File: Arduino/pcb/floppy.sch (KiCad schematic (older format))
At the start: 11 parts, among them J7 Floppy-Power, J8 IBM_PC_Floppy_IDC, SW1 Bus Address Select, U1 4021

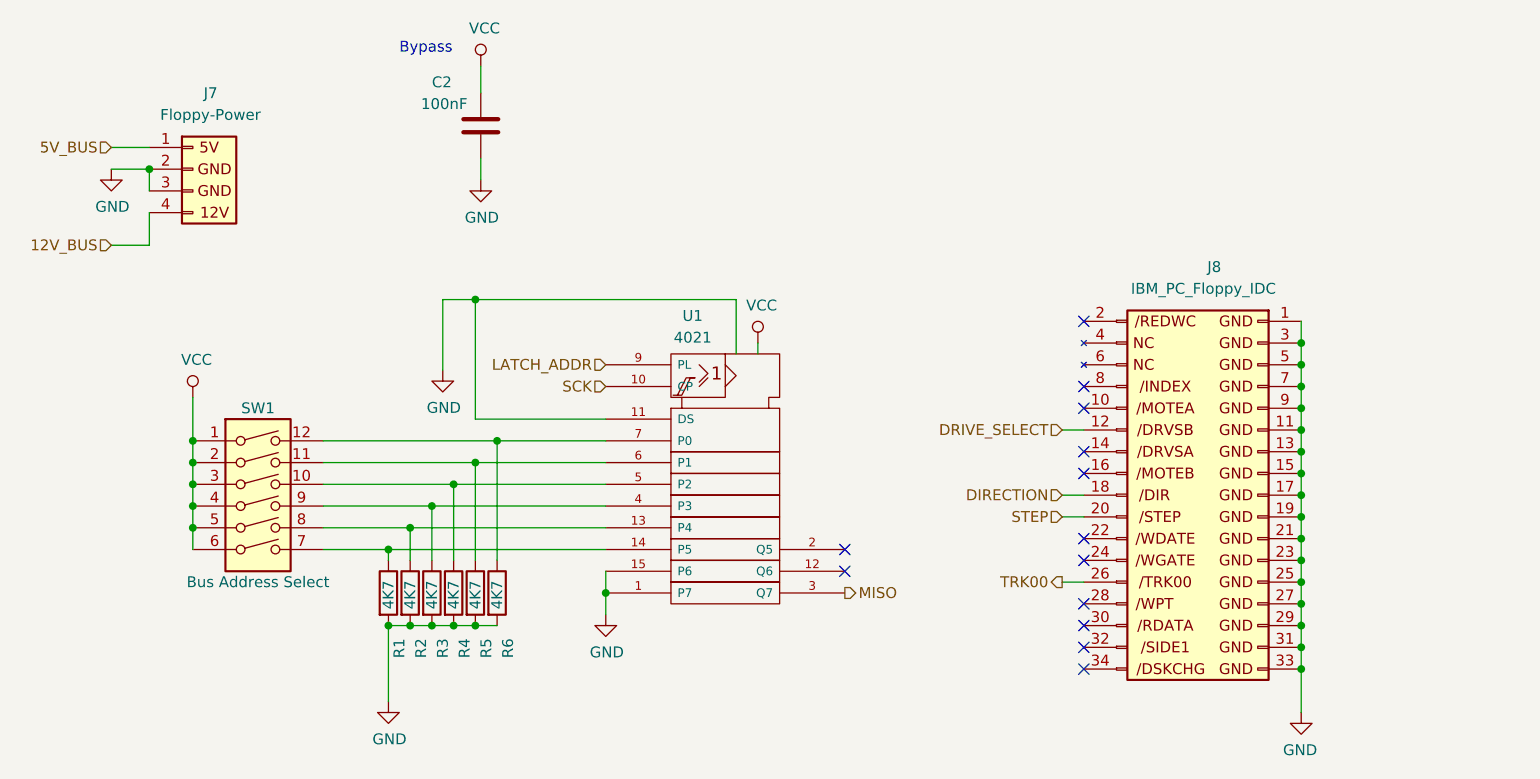
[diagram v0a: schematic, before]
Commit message: pcb: did... something
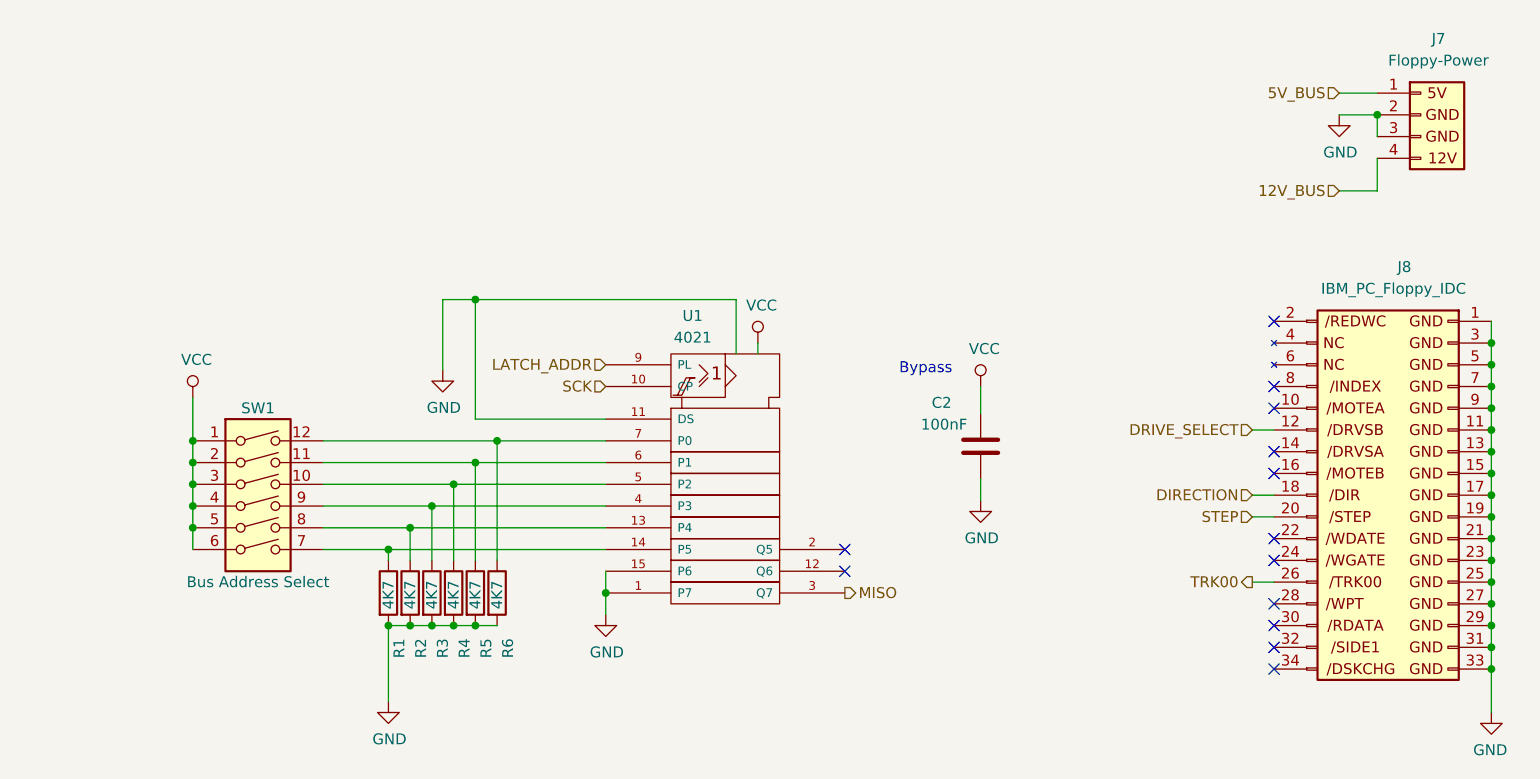
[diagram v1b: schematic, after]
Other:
- moved on the sheet: C2, J7, J8
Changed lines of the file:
@@
 Comment4 ""
 $EndDescr
-NoConn ~ 6075 2925
-NoConn ~ 6075 3025
-NoConn ~ 6075 3325
-NoConn ~ 6075 3625
-NoConn ~ 6075 3725
-NoConn ~ 6075 3925
-NoConn ~ 6075 4025
-NoConn ~ 6075 4125
-NoConn ~ 6075 4225
-NoConn ~ 6075 2625
-NoConn ~ 6075 3225
+NoConn ~ 6950 2925
+NoConn ~ 6950 3025
+NoConn ~ 6950 3325
+NoConn ~ 6950 3625
+NoConn ~ 6950 3725
+NoConn ~ 6950 3925
+NoConn ~ 6950 4025
+NoConn ~ 6950 4125
+NoConn ~ 6950 4225
+NoConn ~ 6950 2625
+NoConn ~ 6950 3225
 $Comp
 L ibm_pc_floppy_idc:IBM_PC_Floppy_IDC J?
 U 1 1 5CE26438
-P 6875 3425
+P 7750 3425
 AR Path="/5CE26438" Ref="J?"  Part="1"
 AR Path="/5CD0EE48/5CE26438" Ref="J8"  Part="1"
-F 0 "J8" H 7075 4475 50  0000 C CNN
-F 1 "IBM_PC_Floppy_IDC" H 7125 4375 50  0000 C CNN
-F 2 "ibm_idc_floppy_connector:ibm_pc_floppy_idc" H 6875 3425 50  0001 C CNN
-F 3 "" H 6875 3425 50  0001 C CNN
-	1    6875 3425
+F 0 "J8" H 7950 4475 50  0000 C CNN
+F 1 "IBM_PC_Floppy_IDC" H 8000 4375 50  0000 C CNN
+F 2 "ibm_idc_floppy_connector:ibm_pc_floppy_idc" H 7750 3425 50  0001 C CNN
+F 3 "" H 7750 3425 50  0001 C CNN
+	1    7750 3425
 	-1   0    0    -1
 $EndComp
 Wire Wire Line
-	7075 2625 7075 2725
-Connection ~ 7075 2725
-Wire Wire Line
-	7075 2725 7075 2825
-Connection ~ 7075 2825
-Wire Wire Line
-	7075 2825 7075 2925
-Connection ~ 7075 2925
-Wire Wire Line
-	7075 2925 7075 3025
-Connection ~ 7075 3025
-Wire Wire Line
-	7075 3025 7075 3125
-Connection ~ 7075 3125
-Wire Wire Line
-	7075 3125 7075 3225
-Connection ~ 7075 3225
-Wire Wire Line
-	7075 3225 7075 3325
-Connection ~ 7075 3325
-Wire Wire Line
-	7075 3325 7075 3425
-Connection ~ 7075 3425
-Wire Wire Line
-	7075 3425 7075 3525
-Connection ~ 7075 3525
-Wire Wire Line
-	7075 3525 7075 3625
-Connection ~ 7075 3625
-Wire Wire Line
-	7075 3625 7075 3725
-Connection ~ 7075 3725
-Wire Wire Line
-	7075 3725 7075 3825
-Connection ~ 7075 3825
-Wire Wire Line
-	7075 3825 7075 3925
-Connection ~ 7075 3925
-Wire Wire Line
-	7075 3925 7075 4025
-Connection ~ 7075 4025
-Wire Wire Line
-	7075 4025 7075 4125
-Wire Wire Line
-	7075 4125 7075 4225
-Connection ~ 7075 4125
-Connection ~ 7075 4225
-Wire Wire Line
-	7075 4225 7075 4425
+	7950 2625 7950 2725
+Connection ~ 7950 2725
+Wire Wire Line
+	7950 2725 7950 2825
+Connection ~ 7950 2825
+Wire Wire Line
+	7950 2825 7950 2925
+Connection ~ 7950 2925
+Wire Wire Line
+	7950 2925 7950 3025
+Connection ~ 7950 3025
+Wire Wire Line
+	7950 3025 7950 3125
+Connection ~ 7950 3125
+Wire Wire Line
+	7950 3125 7950 3225
+Connection ~ 7950 3225
+Wire Wire Line
+	7950 3225 7950 3325
+Connection ~ 7950 3325
+Wire Wire Line
+	7950 3325 7950 3425
+Connection ~ 7950 3425
+Wire Wire Line
+	7950 3425 7950 3525
+Connection ~ 7950 3525
+Wire Wire Line
+	7950 3525 7950 3625
+Connection ~ 7950 3625
+Wire Wire Line
+	7950 3625 7950 3725
+Connection ~ 7950 3725
+Wire Wire Line
+	7950 3725 7950 3825
+Connection ~ 7950 3825
+Wire Wire Line
+	7950 3825 7950 3925
+Connection ~ 7950 3925
+Wire Wire Line
+	7950 3925 7950 4025
+Connection ~ 7950 4025
+Wire Wire Line
+	7950 4025 7950 4125
+Wire Wire Line
+	7950 4125 7950 4225
+Connection ~ 7950 4125
+Connection ~ 7950 4225
+Wire Wire Line
+	7950 4225 7950 4425
 $Comp
 L power:GND #PWR?
 U 1 1 5CE2645F
-P 7075 4425
+P 7950 4425
 AR Path="/5CE2645F" Ref="#PWR?"  Part="1"
 AR Path="/5CD0EE48/5CE2645F" Ref="#PWR018"  Part="1"
-F 0 "#PWR018" H 7075 4175 50  0001 C CNN
-F 1 "GND" H 7080 4252 50  0000 C CNN
-F 2 "" H 7075 4425 50  0001 C CNN
-F 3 "" H 7075 4425 50  0001 C CNN
-	1    7075 4425
+F 0 "#PWR018" H 7950 4175 50  0001 C CNN
+F 1 "GND" H 7955 4252 50  0000 C CNN
+F 2 "" H 7950 4425 50  0001 C CNN
+F 3 "" H 7950 4425 50  0001 C CNN
+	1    7950 4425
 	-1   0    0    -1
 $EndComp
-Text HLabel 5975 3125 0    50   Input ~ 0
+Text HLabel 6850 3125 0    50   Input ~ 0
 DRIVE_SELECT
-Text HLabel 5975 3425 0    50   Input ~ 0
+Text HLabel 6850 3425 0    50   Input ~ 0
 DIRECTION
-Text HLabel 5975 3825 0    50   Output ~ 0
+Text HLabel 6850 3825 0    50   Output ~ 0
 TRK00
-Text HLabel 5975 3525 0    50   Input ~ 0
+Text HLabel 6850 3525 0    50   Input ~ 0
 STEP
 Wire Wire Line
-	5975 3125 6075 3125
-Wire Wire Line
-	5975 3425 6075 3425
-Wire Wire Line
-	5975 3525 6075 3525
-Wire Wire Line
-	5975 3825 6075 3825
+	6850 3125 6950 3125
+Wire Wire Line
+	6850 3425 6950 3425
+Wire Wire Line
+	6850 3525 6950 3525
+Wire Wire Line
+	6850 3825 6950 3825
 $Comp
 L floppy-power:Floppy-Power J?
 U 1 1 5CEBDDC6
-P 1975 1925
+P 7625 1675
 AR Path="/5CEBDDC6" Ref="J?"  Part="1"
 AR Path="/5CD0EE48/5CEBDDC6" Ref="J7"  Part="1"
-F 0 "J7" H 2025 2275 50  0000 L CNN
-F 1 "Floppy-Power" H 1825 2175 50  0000 L CNN
-F 2 "floppy_power:Floppy_Power_1x04_Pitch2.54mm" H 1975 1925 50  0001 C CNN
-F 3 "" H 1975 1925 50  0001 C CNN
-	1    1975 1925
+F 0 "J7" H 7675 2025 50  0000 L CNN
+F 1 "Floppy-Power" H 7475 1925 50  0000 L CNN
+F 2 "floppy_power:Floppy_Power_1x04_Pitch2.54mm" H 7625 1675 50  0001 C CNN
+F 3 "" H 7625 1675 50  0001 C CNN
+	1    7625 1675
 	1    0    0    -1
 $EndComp
@@
 L power:GND #PWR?
 U 1 1 5CEBDDD4
-P 1600 1925
+P 7250 1675
 AR Path="/5CEBDDD4" Ref="#PWR?"  Part="1"
 AR Path="/5CD0EE48/5CEBDDD4" Ref="#PWR010"  Part="1"
-F 0 "#PWR010" H 1600 1675 50  0001 C CNN
-F 1 "GND" H 1605 1752 50  0000 C CNN
-F 2 "" H 1600 1925 50  0001 C CNN
-F 3 "" H 1600 1925 50  0001 C CNN
-	1    1600 1925
-	1    0    0    -1
-$EndComp
-Wire Wire Line
-	1775 2025 1775 1925
-Connection ~ 1775 1925
-Wire Wire Line
-	1600 1925 1775 1925
-Wire Wire Line
-	1775 2275 1775 2125
-Wire Wire Line
-	1600 1825 1775 1825
-Text HLabel 1600 1825 0    50   Input ~ 0
+F 0 "#PWR010" H 7250 1425 50  0001 C CNN
+F 1 "GND" H 7255 1502 50  0000 C CNN
+F 2 "" H 7250 1675 50  0001 C CNN
+F 3 "" H 7250 1675 50  0001 C CNN
+	1    7250 1675
+	1    0    0    -1
+$EndComp
+Wire Wire Line
+	7425 1775 7425 1675
+Connection ~ 7425 1675
+Wire Wire Line
+	7250 1675 7425 1675
+Wire Wire Line
+	7425 2025 7425 1875
+Wire Wire Line
+	7250 1575 7425 1575
+Text HLabel 7250 1575 0    50   Input ~ 0
 5V_BUS
-Text HLabel 1600 2275 0    50   Input ~ 0
+Text HLabel 7250 2025 0    50   Input ~ 0
 12V_BUS
 Wire Wire Line
-	1600 2275 1775 2275
+	7250 2025 7425 2025
 $Comp
 L floppyorgel-rescue:SW_DIP_x06-switches SW?
@@
 L Device:C C?
 U 1 1 5CD16AEF
-P 3300 1725
+P 5600 3200
 AR Path="/5CD16AEF" Ref="C?"  Part="1"
 AR Path="/5CCFEC3E/5CD16AEF" Ref="C?"  Part="1"
 AR Path="/5CD1E0A5/5CD16AEF" Ref="C?"  Part="1"
 AR Path="/5CD0EE48/5CD16AEF" Ref="C2"  Part="1"
-F 0 "C2" H 3075 1925 50  0000 L CNN
-F 1 "100nF" H 3025 1825 50  0000 L CNN
-F 2 "Capacitor_SMD:C_0805_2012Metric" H 3338 1575 50  0001 C CNN
-F 3 "~" H 3300 1725 50  0001 C CNN
-	1    3300 1725
+F 0 "C2" H 5375 3400 50  0000 L CNN
+F 1 "100nF" H 5325 3300 50  0000 L CNN
+F 2 "Capacitor_SMD:C_0805_2012Metric" H 5638 3050 50  0001 C CNN
+F 3 "~" H 5600 3200 50  0001 C CNN
+	1    5600 3200
 	1    0    0    -1
 $EndComp
@@
 L power:VCC #PWR?
 U 1 1 5CD16AF5
-P 3300 1450
+P 5600 2925
 AR Path="/5CCFEC3E/5CD16AF5" Ref="#PWR?"  Part="1"
 AR Path="/5CD1E0A5/5CD16AF5" Ref="#PWR?"  Part="1"
 AR Path="/5CD0EE48/5CD16AF5" Ref="#PWR014"  Part="1"
-F 0 "#PWR014" H 3300 1300 50  0001 C CNN
-F 1 "VCC" H 3317 1623 50  0000 C CNN
-F 2 "" H 3300 1450 50  0001 C CNN
-F 3 "" H 3300 1450 50  0001 C CNN
-	1    3300 1450
+F 0 "#PWR014" H 5600 2775 50  0001 C CNN
+F 1 "VCC" H 5617 3098 50  0000 C CNN
+F 2 "" H 5600 2925 50  0001 C CNN
+F 3 "" H 5600 2925 50  0001 C CNN
+	1    5600 2925
 	1    0    0    -1
 $EndComp
@@
 L power:GND #PWR?
 U 1 1 5CD16AFB
-P 3300 1975
+P 5600 3450
 AR Path="/5CCFEC3E/5CD16AFB" Ref="#PWR?"  Part="1"
 AR Path="/5CD1E0A5/5CD16AFB" Ref="#PWR?"  Part="1"
 AR Path="/5CD0EE48/5CD16AFB" Ref="#PWR015"  Part="1"
-F 0 "#PWR015" H 3300 1725 50  0001 C CNN
-F 1 "GND" H 3305 1802 50  0000 C CNN
-F 2 "" H 3300 1975 50  0001 C CNN
-F 3 "" H 3300 1975 50  0001 C CNN
-	1    3300 1975
-	1    0    0    -1
-$EndComp
-Wire Wire Line
-	3300 1450 3300 1575
-Wire Wire Line
-	3300 1875 3300 1975
-Text Notes 2925 1400 0    50   ~ 0
+F 0 "#PWR015" H 5600 3200 50  0001 C CNN
+F 1 "GND" H 5605 3277 50  0000 C CNN
+F 2 "" H 5600 3450 50  0001 C CNN
+F 3 "" H 5600 3450 50  0001 C CNN
+	1    5600 3450
+	1    0    0    -1
+$EndComp
+Wire Wire Line
+	5600 2925 5600 3050
+Wire Wire Line
+	5600 3350 5600 3450
+Text Notes 5225 2875 0    50   ~ 0
 Bypass
 $EndSCHEMATC
